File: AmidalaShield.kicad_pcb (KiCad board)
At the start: 4 copper layers, 106 x 73 mm, 37 parts, among them J1 Screw_Terminal_01x02, J3 Micro_SD_Card

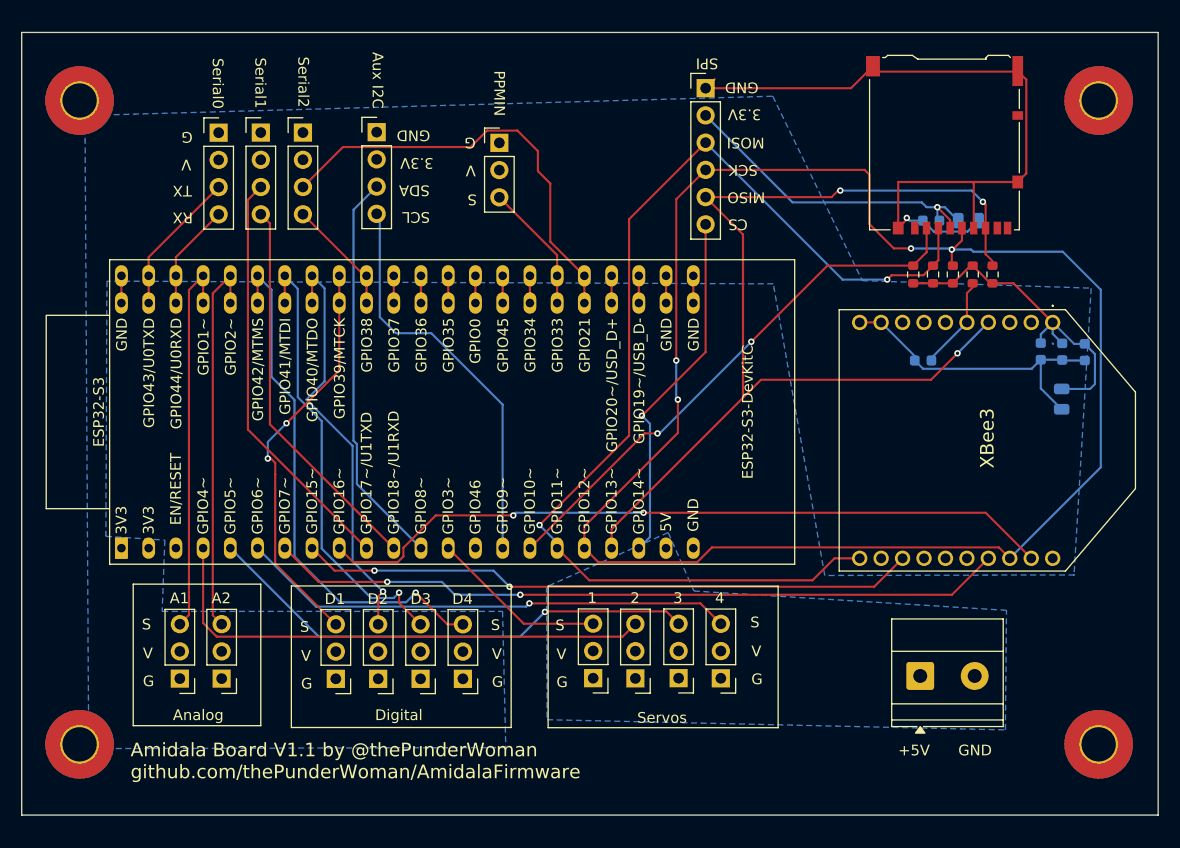
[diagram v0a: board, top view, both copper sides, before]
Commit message: Updated to v1.2 to address remaining issues
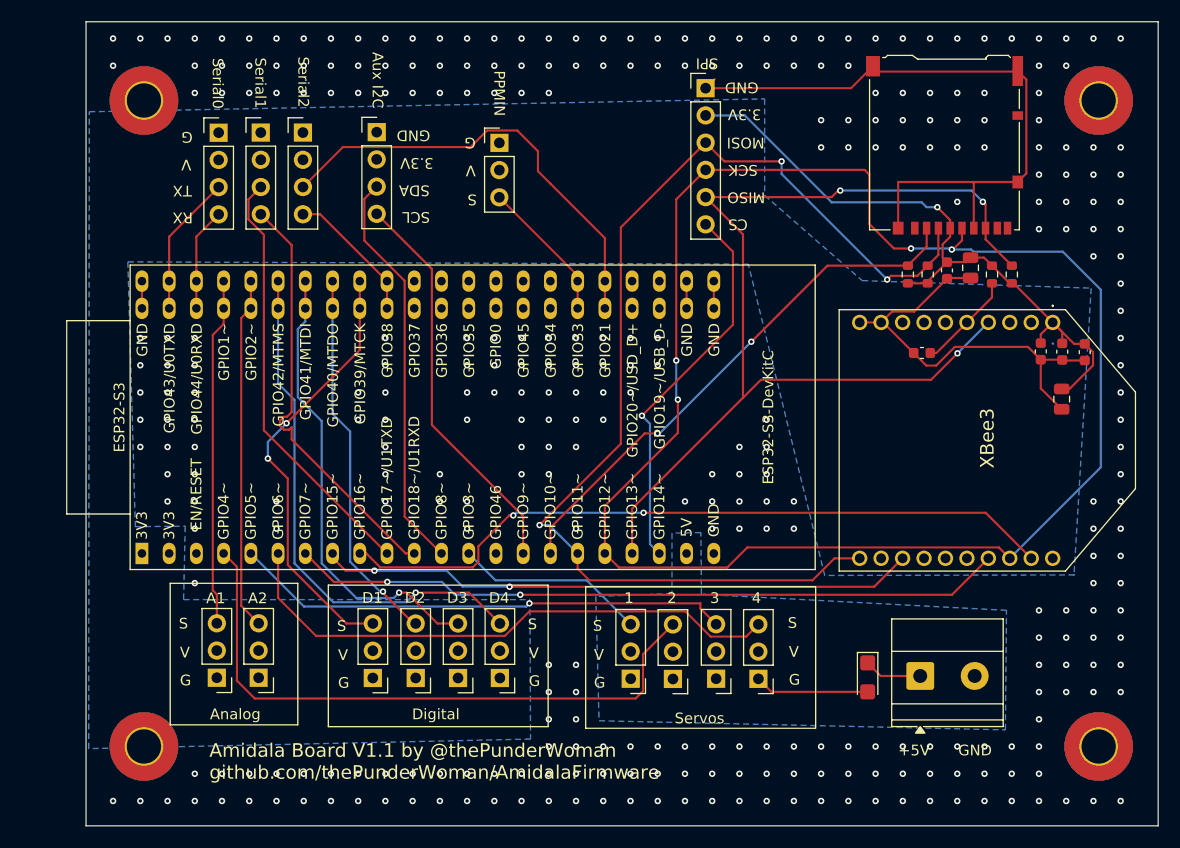
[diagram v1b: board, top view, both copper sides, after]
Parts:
- removed R4: 10k, Resistor_SMD:R_0603_1608Metric
- added C9: 100µF, Capacitor_Tantalum_SMD:CP_EIA-3216-18_Kemet-A, F.Cu at (139.4, 97.2)
- C1, C2, C3, C4, C5, C6, C7: moved to F.Cu
- moved REF** 6.00 mm to (71.9, 103.6)
- moved REF** 6.00 mm to (71.9, 43.4)
- moved C3 4.88 mm to (146.8, 59.2), turned to -90 degrees
- moved C4 4.40 mm to (149.0, 59.0), turned to -90 degrees
- moved J_Digital2 3.50 mm to (97.2, 97.2)
- moved J_Digital3 3.50 mm to (101.2, 97.2)
- moved J_Servo4 3.50 mm to (129.2, 97.3)
- moved J_Servo1 3.50 mm to (117.3, 97.3)
- moved J_Servo2 3.50 mm to (121.2, 97.3)
- moved J_Servo3 3.50 mm to (125.3, 97.3)
- moved J_Analog1 3.45 mm to (78.7, 97.2)
- moved J_Digital1 3.45 mm to (93.2, 97.2)
- moved J_Analog2 3.45 mm to (82.6, 97.2)
- moved J_Digital4 3.45 mm to (105.1, 97.2)
- moved G*** 2.86 mm to (116.2, 72.8)
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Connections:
- ESP32-S3 pad 1: unconnected-(ESP32-S3-3V3-Pad1) -> +3.3V
- ESP32-S3 pad 2: unconnected-(ESP32-S3-3V3-Pad1)_1 -> +3.3V
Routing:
- net GND: track 107.7 -> 120.0 mm, vias 1 -> 333
- net /Servos/GPIO4: track 48.3 -> 58.6 mm
- net /Servos/GPIO6: track 46.4 -> 52.8 mm, vias 1 -> 0
- net +5V: track 0.00 -> 5.41 mm
- net /Pins/GPIO40: track 39.4 -> 35.4 mm
- net /Comms/GPIO18: track 36.3 -> 39.8 mm
- net /SPI/GPIO12: track 158.0 -> 154.5 mm
- net /Pins/GPIO1: track 35.9 -> 32.5 mm
- net /Pins/GPIO2: track 36.1 -> 33.0 mm
- net /Pins/GPIO39: track 38.5 -> 41.3 mm
- net unconnected-(ESP32-S3-GPIO48-Pad29): track 2.54 -> 0.00 mm
- net unconnected-(ESP32-S3-GPIO45-Pad30): track 2.54 -> 0.00 mm
- net unconnected-(ESP32-S3-GPIO37-Pad34)_1: track 2.54 -> 0.00 mm
- net unconnected-(ESP32-S3-GPIO36-Pad33): track 2.54 -> 0.00 mm
- net unconnected-(ESP32-S3-GPIO35-Pad32)_1: track 2.54 -> 0.00 mm
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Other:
- board size 106 x 73 mm -> 100 x 75 mm
